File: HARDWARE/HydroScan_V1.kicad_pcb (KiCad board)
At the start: 4 copper layers, 202 x 100 mm, 38 parts, among them U1 IP2312-4V35, U13 ESP32-WROOM-32D, U14 CH340C, U15 CH340C, U16 ESP32-WROOM-32D, U2 BQ25798RQMR

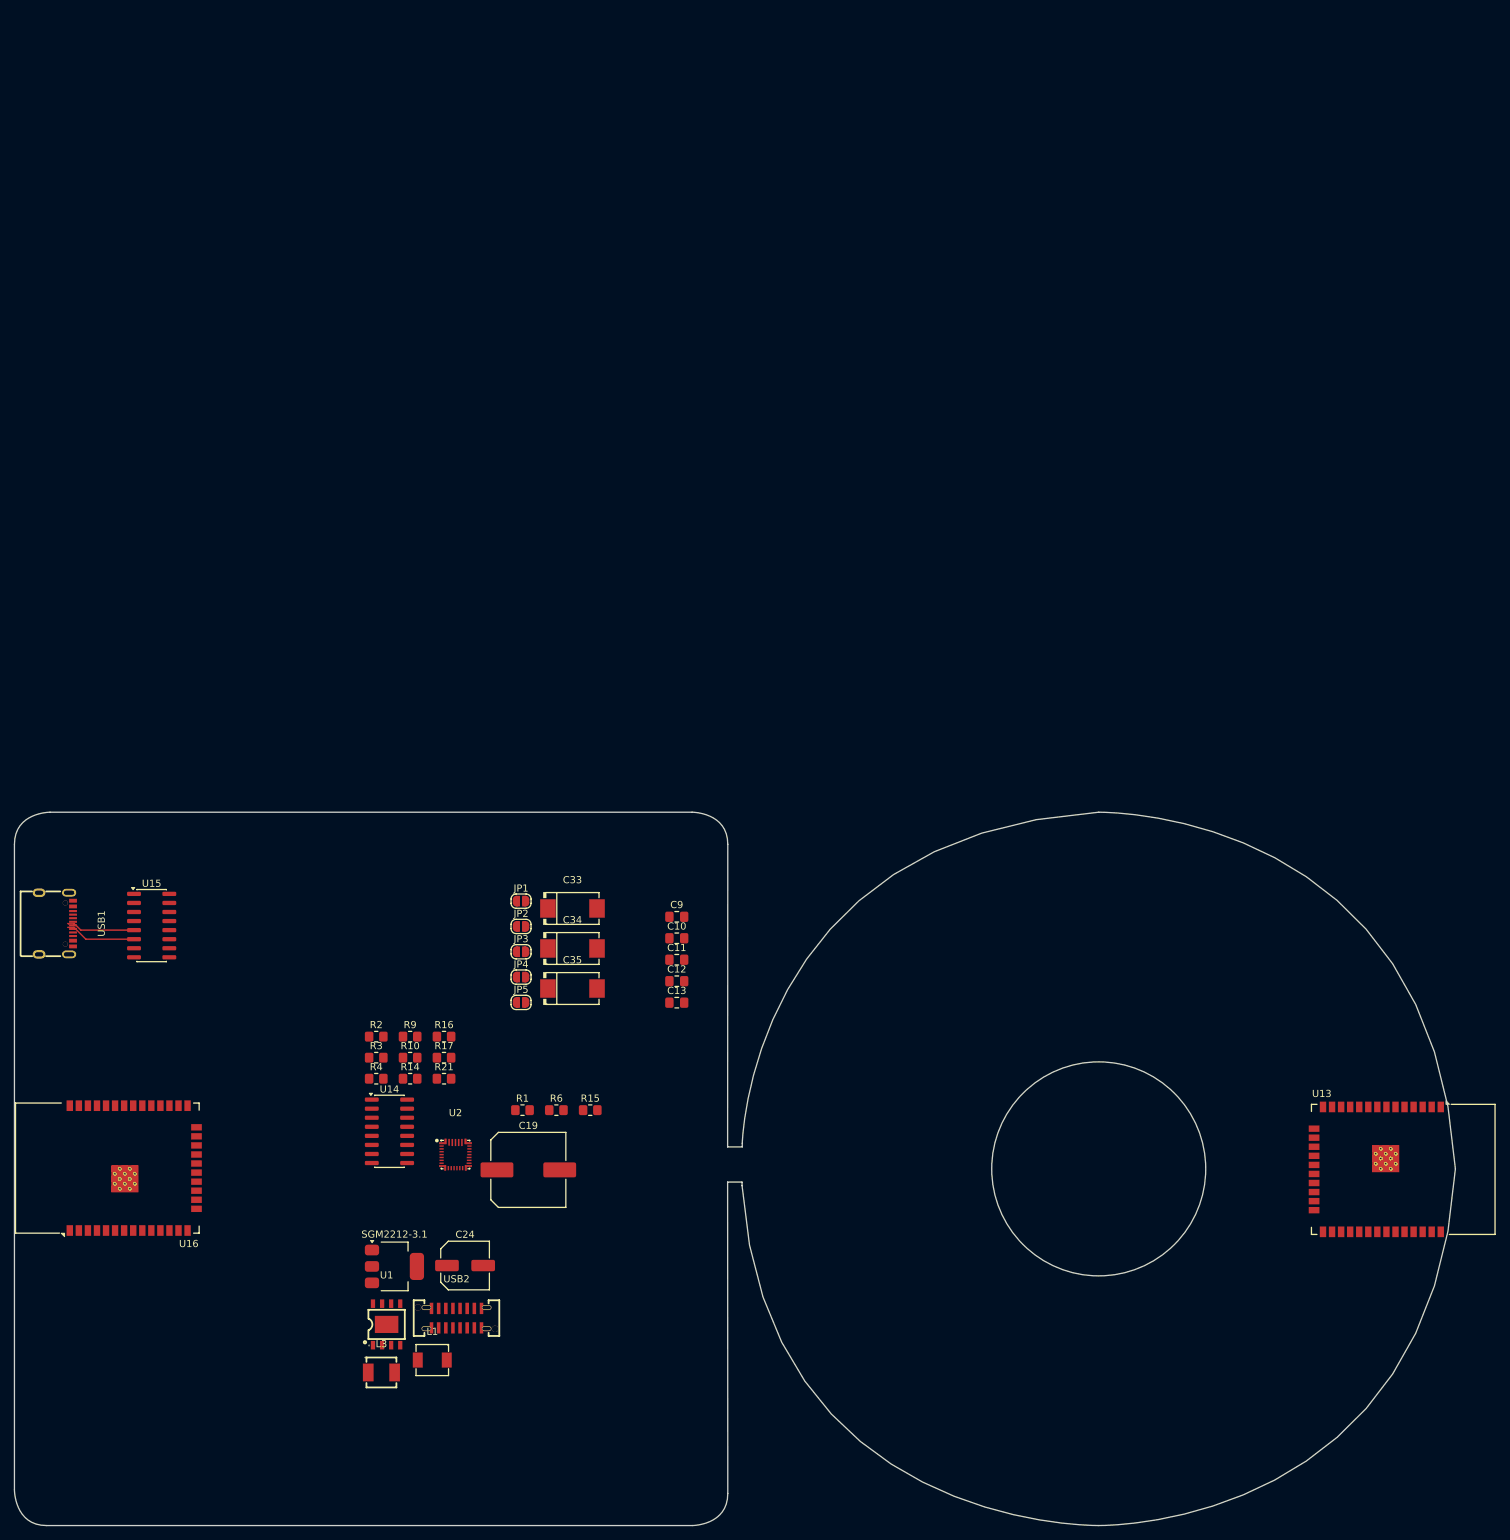
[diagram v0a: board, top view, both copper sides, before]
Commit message: Avances puerto USB C
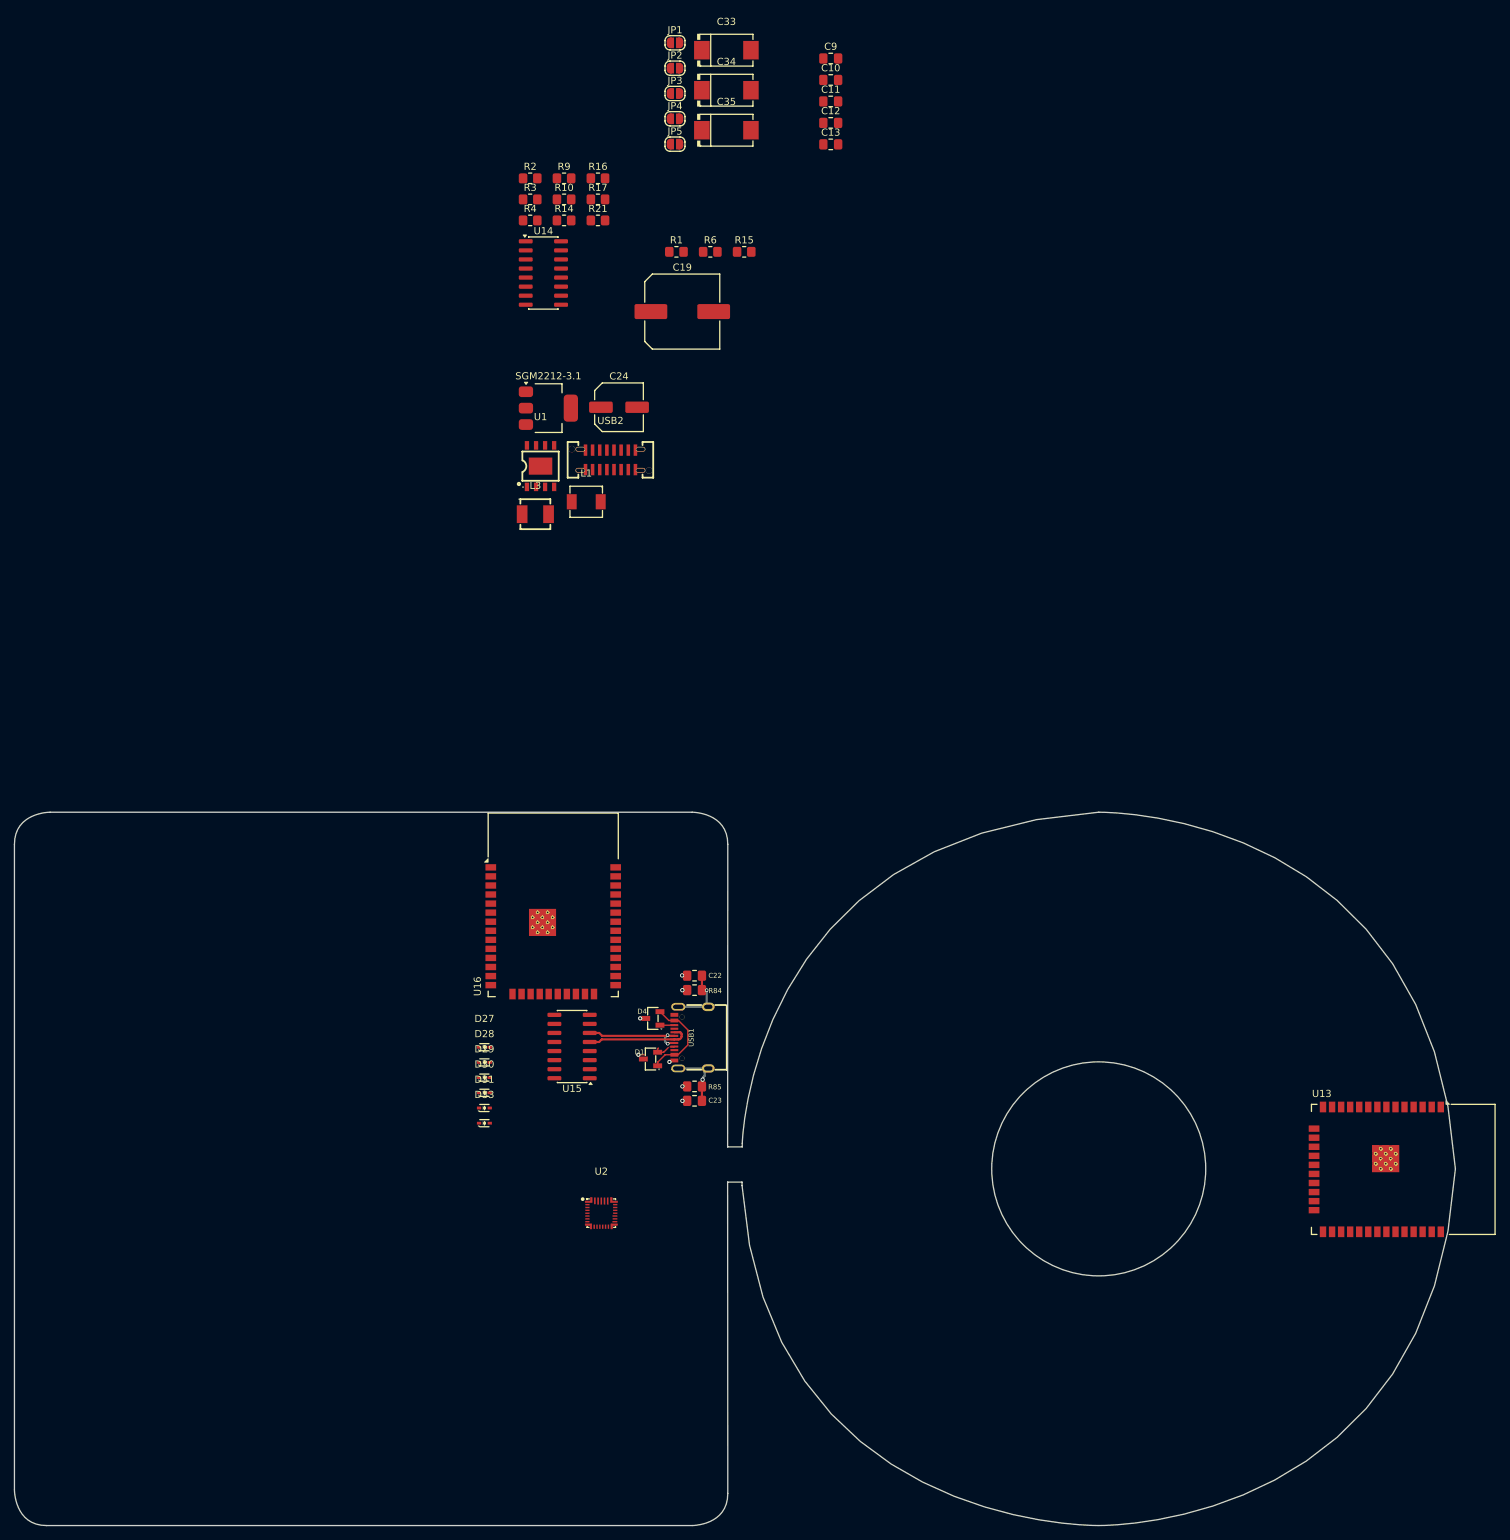
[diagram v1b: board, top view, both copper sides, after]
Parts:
- added C22: 0.1uf, Capacitor_SMD:C_0805_2012Metric_Pad1.18x1.45mm_HandSolder, F.Cu at (175.3, 142.9)
- added C23: 0.1uf, Capacitor_SMD:C_0805_2012Metric_Pad1.18x1.45mm_HandSolder, F.Cu at (175.3, 160.5)
- added D1: SM05.TCT, EasyEDA:SOT-23-3_L2.9-W1.3-P0.95-LS2.4-BR, F.Cu at (169.2, 154.6)
- added D27: LESD5D5.0CT1G, EasyEDA:SOD-523_L1.2-W0.8-LS1.6-BI, F.Cu at (145.9, 152.9)
- added D28: LESD5D5.0CT1G, EasyEDA:SOD-523_L1.2-W0.8-LS1.6-BI, F.Cu at (145.9, 155.1)
- added D29: LESD5D5.0CT1G, EasyEDA:SOD-523_L1.2-W0.8-LS1.6-BI, F.Cu at (145.9, 157.2)
- added D30: LESD5D5.0CT1G, EasyEDA:SOD-523_L1.2-W0.8-LS1.6-BI, F.Cu at (145.9, 159.3)
- added D31: LESD5D5.0CT1G, EasyEDA:SOD-523_L1.2-W0.8-LS1.6-BI, F.Cu at (145.9, 161.5)
- added D33: LESD5D5.0CT1G, EasyEDA:SOD-523_L1.2-W0.8-LS1.6-BI, F.Cu at (145.9, 163.6)
- added D4: SM05.TCT, EasyEDA:SOT-23-3_L2.9-W1.3-P0.95-LS2.4-BR, F.Cu at (169.5, 148.9)
- added R84: 1M, Capacitor_SMD:C_0805_2012Metric_Pad1.18x1.45mm_HandSolder, F.Cu at (175.3, 144.9)
- added R85: 1M, Capacitor_SMD:C_0805_2012Metric_Pad1.18x1.45mm_HandSolder, F.Cu at (175.3, 158.4)
- moved C24 122.2 mm to (164.8, 63.2)
- moved R14 122.2 mm to (157.1, 37.0)
- moved R21 122.2 mm to (161.8, 37.0)
- moved R4 122.2 mm to (152.3, 37.0)
- moved SGM2212-3.1 122.2 mm to (154.8, 63.4)
- moved U14 122.2 mm to (154.2, 44.4)
- moved C11 122.2 mm to (194.4, 20.4)
- moved C33 122.2 mm to (179.8, 13.2)
- moved C35 122.2 mm to (179.8, 24.4)
- moved JP1 122.2 mm to (172.6, 12.1)
- moved JP4 122.2 mm to (172.6, 22.8)
- moved L1 122.2 mm to (160.2, 76.5)
- moved R16 122.2 mm to (161.8, 31.1)
- moved R2 122.2 mm to (152.3, 31.1)
- moved R9 122.2 mm to (157.1, 31.1)
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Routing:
- net /V5_1: track 0.00 -> 12.8 mm
- net Net-(C22-Pad1): track 0.00 -> 9.76 mm, vias 0 -> 1
- net Net-(C23-Pad1): track 0.00 -> 9.12 mm, vias 0 -> 1
- net GND: track 0.00 -> 5.07 mm, vias 0 -> 7
- net /Data+_1: track 9.71 -> 14.7 mm
- net /Data-_1: track 9.98 -> 14.6 mm, vias 0 -> 2
- net /CC1_1: track 0.00 -> 3.02 mm
- net /CC2_1: track 0.00 -> 2.01 mm
